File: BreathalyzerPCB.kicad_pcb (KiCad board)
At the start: 2 copper layers, 44.5 x 54.6 mm, 19 parts, among them J101 Power Switch, J102 Battery, J103 RGBConn, J104 Read LED, J105 MQ3, U101 MAX6105, U102 ABX00030

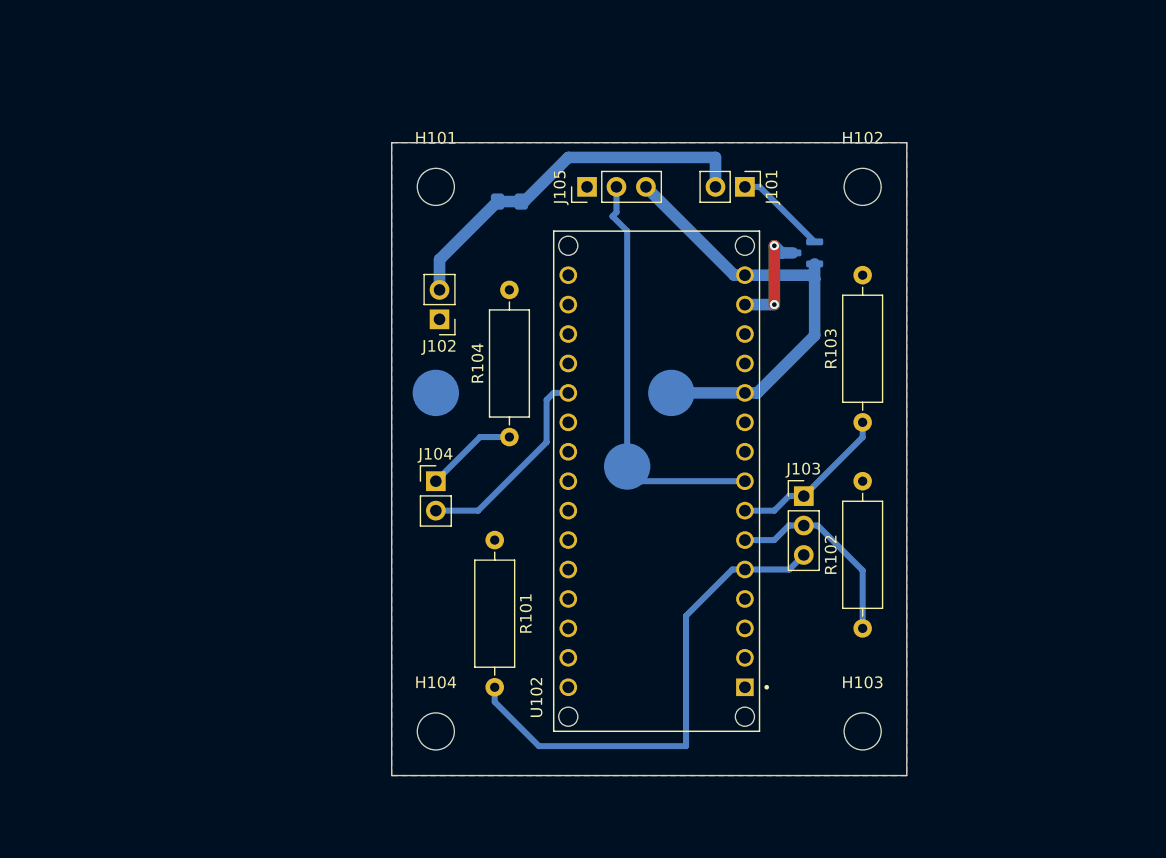
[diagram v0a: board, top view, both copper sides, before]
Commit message: v3.1.0
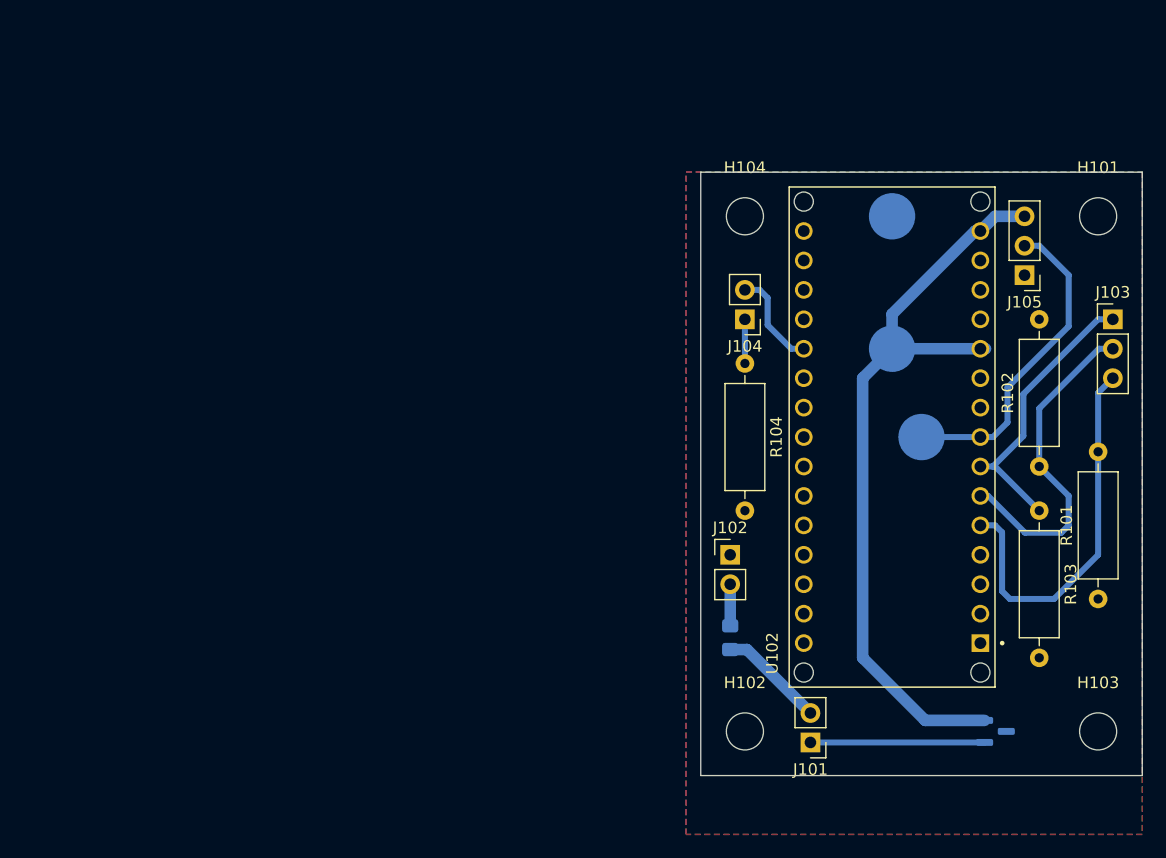
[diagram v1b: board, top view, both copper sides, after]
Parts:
- moved H101 57.2 mm to (194.3, 83.8)
- moved R101 52.3 mm to (194.3, 116.8), turned to 90 degrees
- moved H104 51.8 mm to (163.8, 83.8)
- moved J101 48.3 mm to (169.5, 129.2), turned to 180 degrees
- moved H102 48.1 mm to (163.8, 128.3)
- moved U101 44.5 mm to (185.4, 128.3), turned to 0 degrees
- moved TP101 42.2 mm to (176.5, 83.8), turned to 180 degrees
- moved F101 42.2 mm to (162.6, 120.2), turned to -90 degrees
- moved J105 38.5 mm to (188.0, 88.9), turned to 180 degrees
- moved J102 32.3 mm to (162.6, 113.0), turned to 0 degrees
- moved J103 30.7 mm to (195.6, 92.7)
- moved J104 30.1 mm to (163.8, 92.7), turned to 180 degrees
- moved TP102 25.5 mm to (179.1, 102.9)
- moved R104 21.3 mm to (163.8, 96.5), turned to -90 degrees
- moved U102 20.7 mm to (176.5, 102.9)
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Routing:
- net VCC: track 38.5 -> 66.5 mm
- net +6V: track 32.6 -> 12.8 mm
- net /BattLED2: track 17.3 -> 28.8 mm
- net /BattLED3: track 14.1 -> 24.4 mm
- net /BattLED1: track 42.9 -> 33.1 mm
- net GND: track 9.48 -> 0.00 mm, vias 2 -> 0
- net /ReadLED: track 17.8 -> 8.56 mm
- net /MQ3Analog: track 35.5 -> 27.7 mm
- net /Switch: track 7.99 -> 15.0 mm
- net Net-(D102-Pad1): track 7.93 -> 3.81 mm
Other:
- board size 44.5 x 54.6 mm -> 38.1 x 52.1 mm

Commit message: v4.1.0
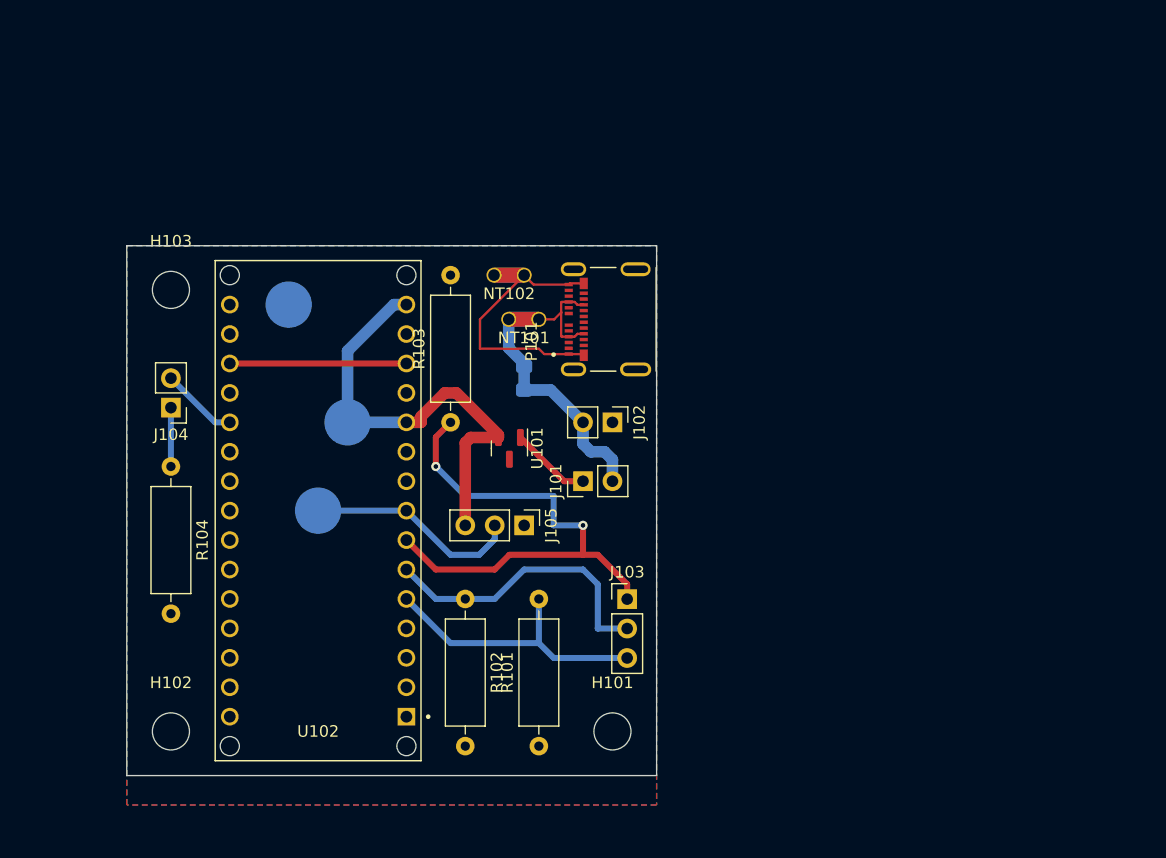
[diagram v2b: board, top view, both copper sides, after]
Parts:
- removed H104: MountingHole, MountingHole:MountingHole_3.2mm_M3
- added NT101: USB_Volt, NetTie:NetTie-2_THT_Pad1.0mm, F.Cu at (146.1, 92.7)
- added NT102: USB_GND, NetTie:NetTie-2_THT_Pad1.0mm, F.Cu at (144.8, 88.9)
- added P101: USBC, 105450-0101:MOLEX_105450-0101, F.Cu at (152.4, 92.7)
- U101: moved to F.Cu
- moved H103 88.6 mm to (114.3, 90.2)
- moved H101 61.1 mm to (152.4, 128.3)
- moved TP101 52.6 mm to (124.5, 91.4)
- moved TP102 52.5 mm to (127.0, 109.2)
- moved R103 51.4 mm to (138.4, 101.6), turned to 90 degrees
- moved R102 50.8 mm to (139.7, 116.8), turned to -90 degrees
- moved R104 50.3 mm to (114.3, 105.4)
- moved J104 50.1 mm to (114.3, 100.3)
- moved U102 49.9 mm to (127.0, 109.2)
- moved R101 49.9 mm to (146.1, 129.5)
- moved H102 49.5 mm to (114.3, 128.3)
- moved U101 48.5 mm to (143.5, 103.8), turned to -90 degrees
- moved J103 48.4 mm to (153.7, 116.9)
- moved J105 48.3 mm to (144.8, 110.5), turned to -90 degrees
- moved TP103 47.4 mm to (129.5, 101.6)
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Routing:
- net VCC: track 66.5 -> 39.2 mm
- net /USBC-GND: track 0.00 -> 22.6 mm
- net /BattLED3: track 24.4 -> 46.1 mm, vias 0 -> 2
- net unconnected-(U102-Pad13): track 0.00 -> 15.2 mm
- net /USBC: track 0.00 -> 9.23 mm
- net /MQ3Analog: track 27.7 -> 18.6 mm
- net /BattLED1: track 33.1 -> 25.0 mm
- net /Switch: track 15.0 -> 6.96 mm
- net +6V: track 12.8 -> 19.7 mm
- net /BattLED2: track 28.8 -> 25.5 mm
- net /ReadLED: track 8.56 -> 6.66 mm
- net Net-(D102-Pad1): track 3.81 -> 5.08 mm
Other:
- board size 38.1 x 52.1 mm -> 45.7 x 45.7 mm

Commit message: v4.4.0
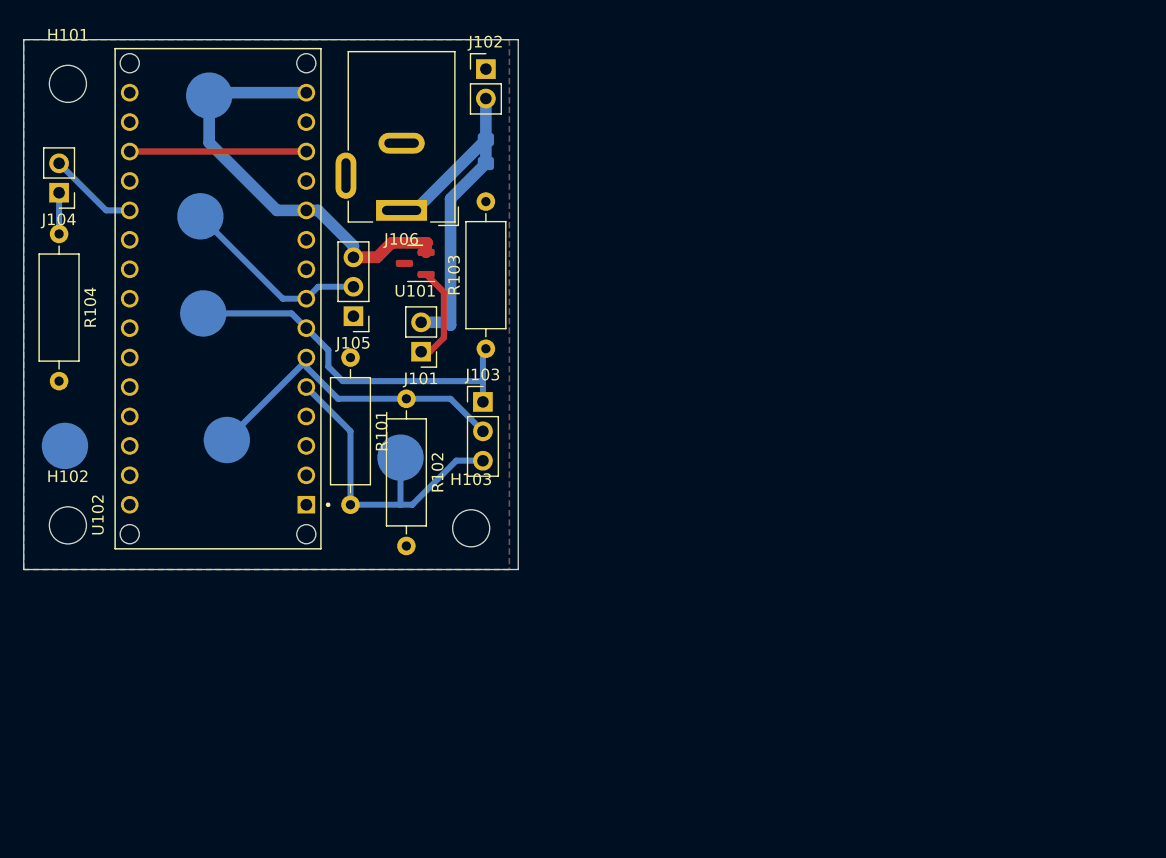
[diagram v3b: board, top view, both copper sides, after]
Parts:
- removed NT101: USB_Volt, NetTie:NetTie-2_THT_Pad1.0mm
- removed NT102: USB_GND, NetTie:NetTie-2_THT_Pad1.0mm
- removed P101: USBC, 105450-0101:MOLEX_105450-0101
- added J106: Barrel_Jack_Switch, Connector_BarrelJack:BarrelJack_Wuerth_6941xx301002, F.Cu at (134.2, 83.3)
- added TP104: BattLED1Test, TestPoint:TestPoint_Pad_D4.0mm, B.Cu at (134.1, 104.6)
- added TP105: BattLED2Test, TestPoint:TestPoint_Pad_D4.0mm, B.Cu at (119.1, 103.1)
- added TP106: BattLED3Test, TestPoint:TestPoint_Pad_D4.0mm, B.Cu at (117.1, 92.2)
- moved H101 73.0 mm to (105.4, 72.4)
- moved R101 37.3 mm to (129.8, 96.0), turned to -90 degrees
- moved H103 33.1 mm to (140.2, 110.7)
- moved J102 32.4 mm to (141.5, 71.1), turned to 0 degrees
- moved TP103 30.6 mm to (117.6, 73.4)
- moved TP102 27.4 mm to (116.8, 83.8)
- moved J105 23.3 mm to (130.0, 92.4), turned to 180 degrees
- moved TP101 22.8 mm to (105.2, 103.6)
- moved R104 22.3 mm to (104.6, 85.3)
- moved J103 21.1 mm to (141.2, 99.8)
- moved J104 20.9 mm to (104.6, 81.8)
- moved U102 20.2 mm to (118.4, 90.9)
- moved H102 19.9 mm to (105.4, 110.5)
- moved F101 19.8 mm to (141.5, 78.2)
- moved R102 18.0 mm to (134.6, 99.6)
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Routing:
- net /USBC-GND: track 22.6 -> 0.00 mm
- net /BattLED3: track 46.1 -> 32.1 mm, vias 2 -> 0
- net +6V: track 19.7 -> 33.3 mm
- net /USBC: track 9.23 -> 0.00 mm
- net /BattLED1: track 25.0 -> 28.8 mm
- net /BattLED2: track 25.5 -> 28.3 mm
- net /MQ3Analog: track 18.6 -> 16.6 mm
- net VCC: track 39.2 -> 37.4 mm
- net /Switch: track 6.96 -> 8.56 mm
- net Net-(D102-Pad1): track 5.08 -> 3.56 mm
- net /ReadLED: track 6.66 -> 7.78 mm
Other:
- board size 45.7 x 45.7 mm -> 42.7 x 45.7 mm
